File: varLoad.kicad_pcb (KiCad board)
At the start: 2 copper layers, 10 parts, among them Q1 MTP3055

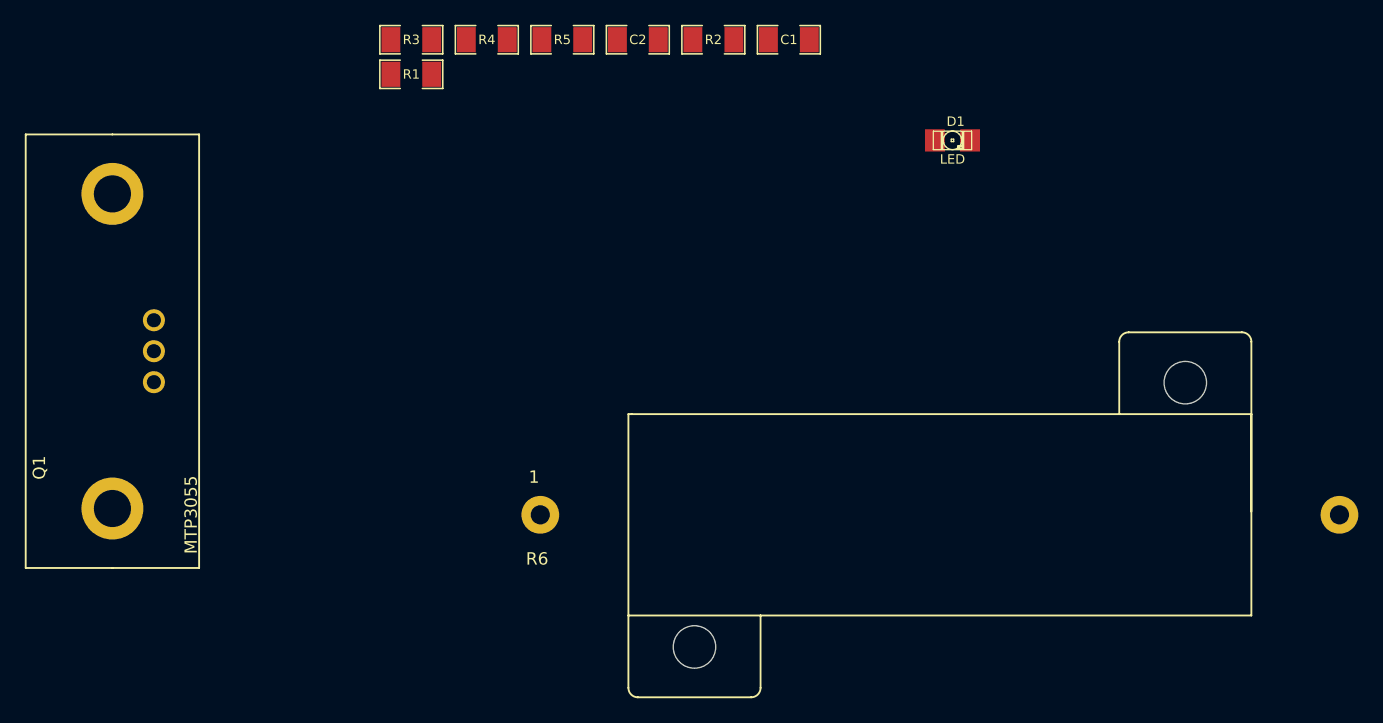
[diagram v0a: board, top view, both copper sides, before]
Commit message: started placement
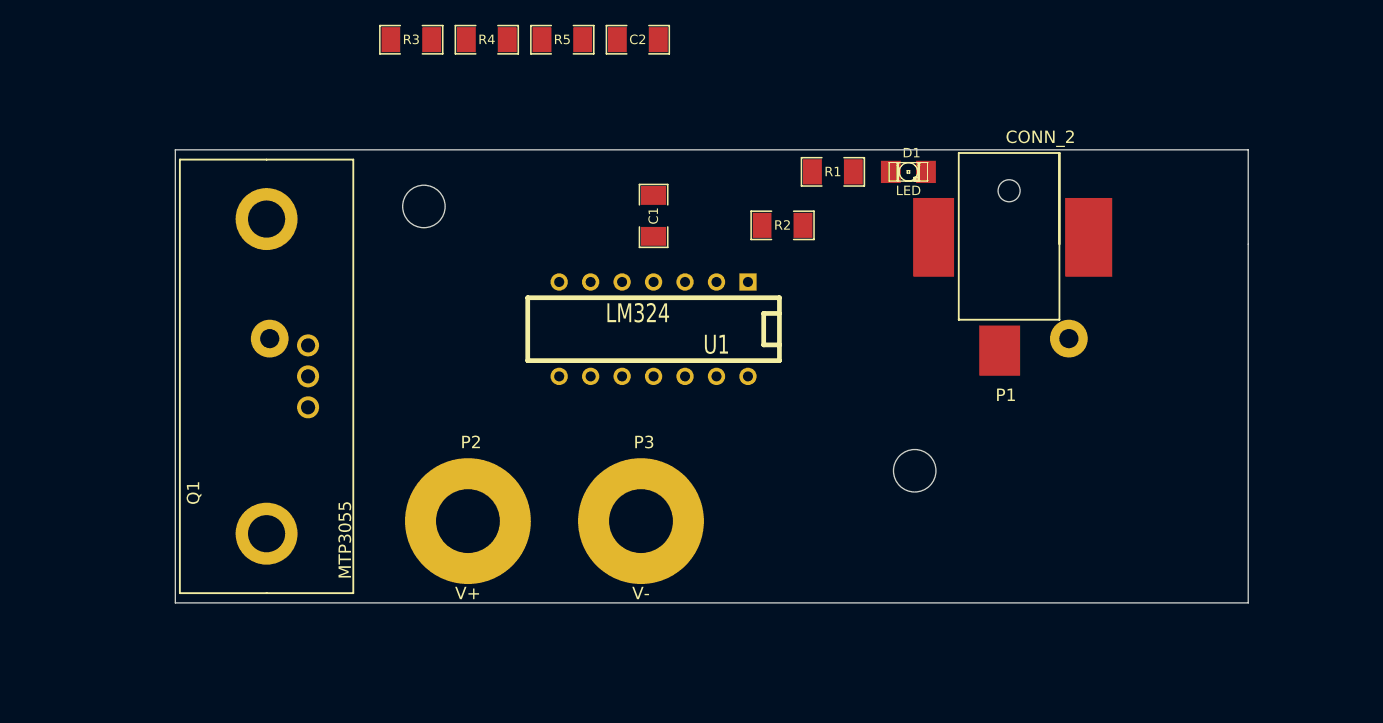
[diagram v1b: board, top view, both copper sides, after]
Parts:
- added P1: CONN_2, RASM722_PowerJack, F.Cu at (159.8, 191.8)
- added P2: V+, bindingPost, F.Cu at (116.1, 218.4)
- added P3: V-, bindingPost, F.Cu at (130.0, 218.4)
- added U1: LM324, DIP-14__300, F.Cu at (131.1, 202.9)
- C1: value C -> 0.1u
- R6: moved to B.Cu
- moved R6 41.7 mm to (112.5, 193.0)
- moved R1 34.9 mm to (145.5, 190.2), turned to 180 degrees
- moved C1 17.9 mm to (131.1, 193.8), turned to 90 degrees
- moved R2 16.0 mm to (141.5, 194.6)
- moved Q1 12.6 mm to (99.8, 219.5)
- moved D1 4.37 mm to (151.6, 190.2)
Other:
- board outline added: 86.6 x 36.6 mm
- board text added: "ADD MOUNTING HOLES"
